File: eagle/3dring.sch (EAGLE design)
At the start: 12 parts, among them U1 Tiny45-20-SMT, U2 NCP1402

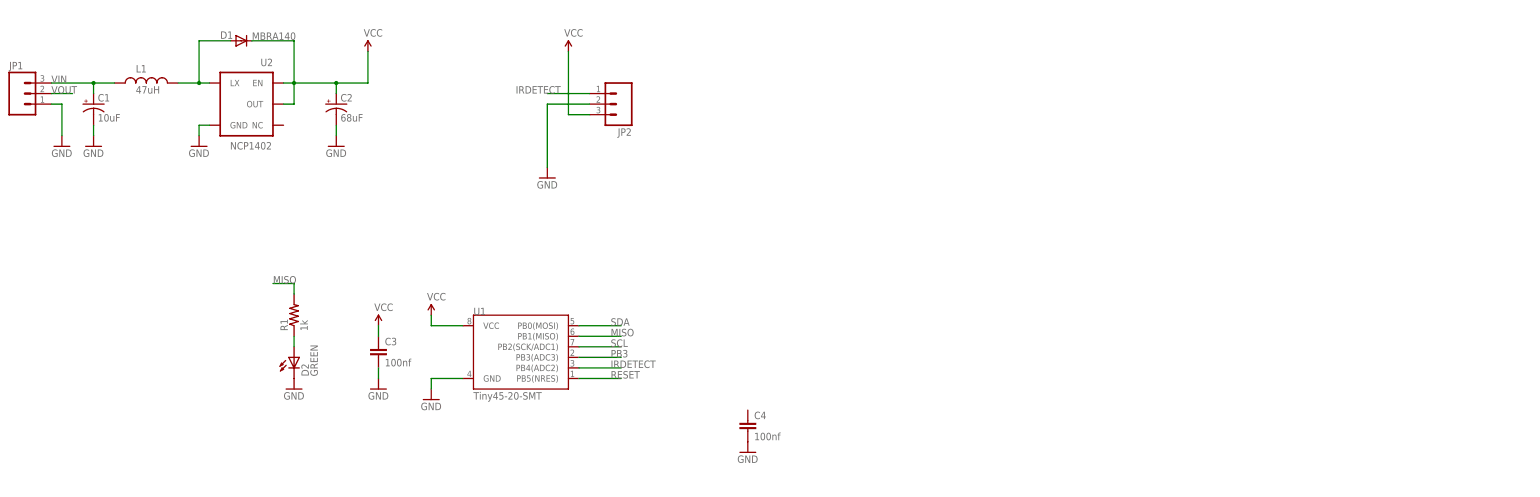
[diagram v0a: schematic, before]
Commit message: board file added and ordered
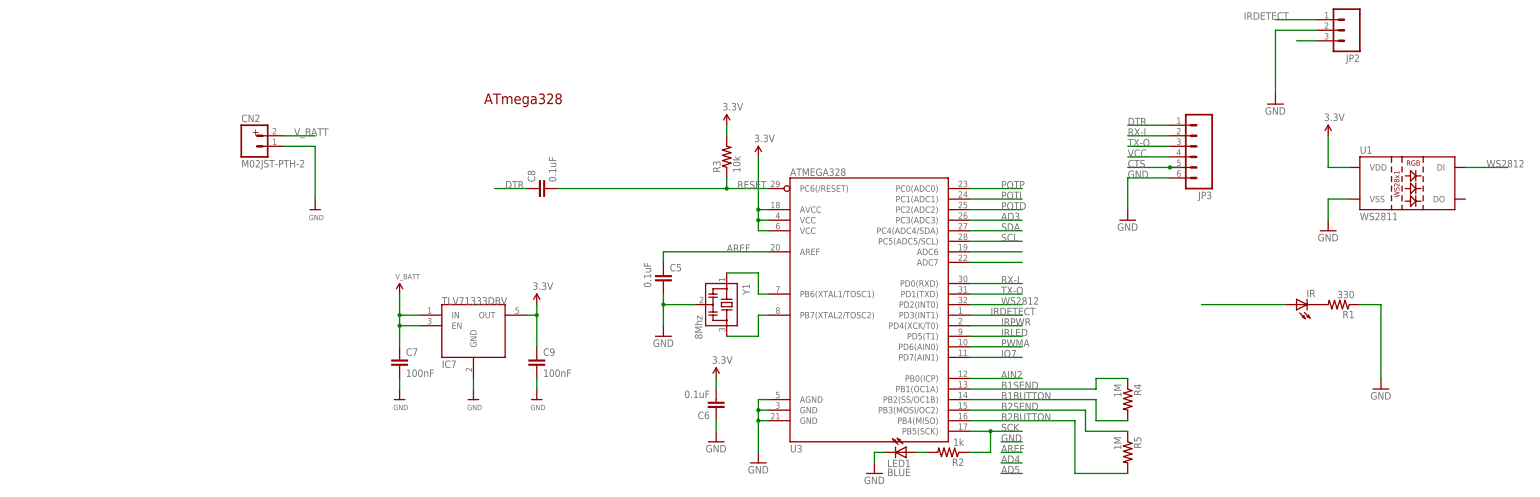
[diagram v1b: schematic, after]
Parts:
- removed C1: 10uF, SparkFun:CAP_POL1206
- removed C2: 68uF, SparkFun:CAP_POL3528
- removed C3, C4: 100nf, SparkFun-Passives:CAP0603-CAP
- removed D1: MBRA140, SparkFun:DIODESMA
- removed D2: GREEN, SparkFun-LED:LED-GREEN0603
- removed JP1: (no value), SparkFun:M03PTH
- removed L1: 47uH, SparkFun:INDUCTORCR54
- removed U2: NCP1402, SparkFun:V_REG_NCP1400SOT23-5
- added C5, C6, C8: 0.1uF, SparkFun:CAP0402-CAP
- added C7, C9: 100nF, rcl:C-EUC0402
- added CN2: M02JST-PTH-2, SparkFun-Connectors:M02JST-PTH-2
- added IC7: TLV71333DBV, anoven:TLV71333DBV
- added IR: (no value), SparkFun-LED:LED5MM
- added JP3: (no value), SparkFun-Connectors:M06SMD-1MM
- added LED1: BLUE, SparkFun:LED0603
- added R2: 1k, SparkFun:RESISTOR0402-RES
- added R3: 10k, SparkFun:RESISTOR0402-RES
- added R4, R5: 1M, SparkFun:RESISTOR0402-RES
- added U3: ATMEGA328, SparkFun:ATMEGA168
- added Y1: 8Mhz, murata-filter:CSTCR6M00G53Z
- R1: value 1k -> 330; device SparkFun-Passives:RESISTOR0603-RES -> SparkFun:RESISTOR0402-RES
- U1: value Tiny45-20-SMT -> WS2811; device SparkFun-DigitalIC:ATTINY45TINY45-20-SMT -> SparkFun-LED:LED-TRICOLOR-5050-ICWS2811
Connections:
- removed net MISO: R1.2, U1.PB1(MISO)
- removed net PB3: U1.PB3(ADC3)
- removed net VIN: C1.+, JP1.3, L1.1
- removed net VOUT: JP1.2
- new net AD3: U3.PC3(ADC3)
- new net AIN2: U3.PB0(ICP)
- new net AREF: C5.1, U3.AREF
- new net B1BUTTON: R4.2, U3.PB2(SS/OC1B)
- new net B1SEND: R4.1, U3.PB1(OC1A)
- new net B2BUTTON: R5.2, U3.PB4(MISO)
- new net B2SEND: R5.1, U3.PB3(MOSI/OC2)
- new net CTS: JP3.5
- new net DTR: C8.1, JP3.1
- new net IO7: U3.PD7(AIN1)
- new net IRLED: IR.A, U3.PD5(T1)
- new net IRPWR: JP2.3, U3.PD4(XCK/T0)
- new net N$1: LED1.A, R2.2
- new net N$4: U3.PB6(XTAL1/TOSC1), Y1.1
- new net N$5: U3.PB7(XTAL2/TOSC2), Y1.3
- new net N$6: U3.ADC7
- new net POTD: U3.PC2(ADC2)
- new net POTI: U3.PC1(ADC1)
- new net POTP: U3.PC0(ADC0)
- new net PWMA: U3.PD6(AIN0)
- new net RX-I: JP3.2, U3.PD0(RXD)
- new net SCK: R2.1, U3.PB5(SCK)
- new net TX-O: JP3.3, U3.PD1(TXD)
- new net V_BATT: C7.1, CN2.2, IC7.EN, IC7.IN
- new net WS2812: U1.DI, U3.PD2(INT0)
- net GND: now also C5.2, C6.1, C7.2, C9.2, CN2.1, IC7.GND, JP3.6, LED1.C, R1.1, U1.VSS, U3.AGND, U3.GND@1, U3.GND@2, Y1.2; no longer C1.-, C2.-, C3.2, C4.2, D2.C, JP1.1, U1.GND, U2.GND
- net IRDETECT: now also U3.PD3(INT1); no longer U1.PB4(ADC2)
- net N$2: now also U3.ADC6; no longer D2.A, R1.1
- net N$3: now also IR.C, R1.2; no longer D1.A, L1.2, U2.LX
- net RESET: now also C8.2, R3.1, U3.PC6(/RESET); no longer U1.PB5(NRES)
- net SCL: now also U3.PC5(ADC5/SCL); no longer U1.PB2(SCK/ADC1)
- net SDA: now also U3.PC4(ADC4/SDA); no longer U1.PB0(MOSI)
- net VCC: now also C6.2, C9.1, IC7.OUT, JP3.4, R3.2, U1.VDD, U3.AVCC, U3.VCC@1, U3.VCC@2; no longer C2.+, C3.1, D1.C, JP2.3, U1.VCC, U2.EN, U2.OUT
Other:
- note added: "ATmega328"
- moved on the sheet: JP2, R1
